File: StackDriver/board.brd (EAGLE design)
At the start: 106.7 x 85.1 mm, 49 parts, among them IC1 LM741P, IC10 LM741P, IC11 LM741P, IC12 LM741P, IC13 LM741P, IC14 LM741P, IC15 LM741P, IC2 LM741P, IC3 LM741P, IC4 LM741P, IC5 LM741P, IC6 LM741P, IC7 LM741P, IC8 LM741P, IC9 LM741P

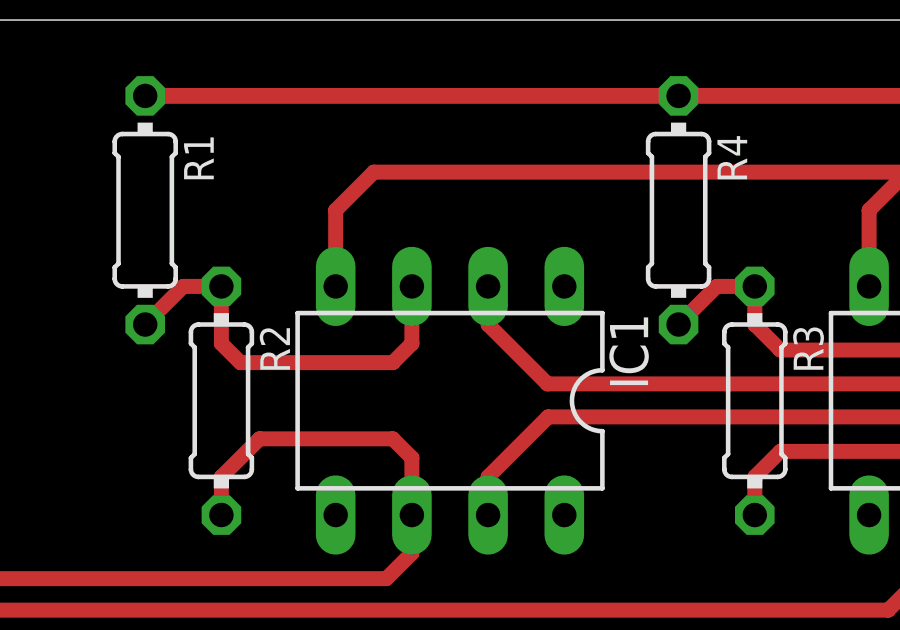
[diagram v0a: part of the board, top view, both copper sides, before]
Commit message: Nie umiem w płytki. Teraz bedzie gut
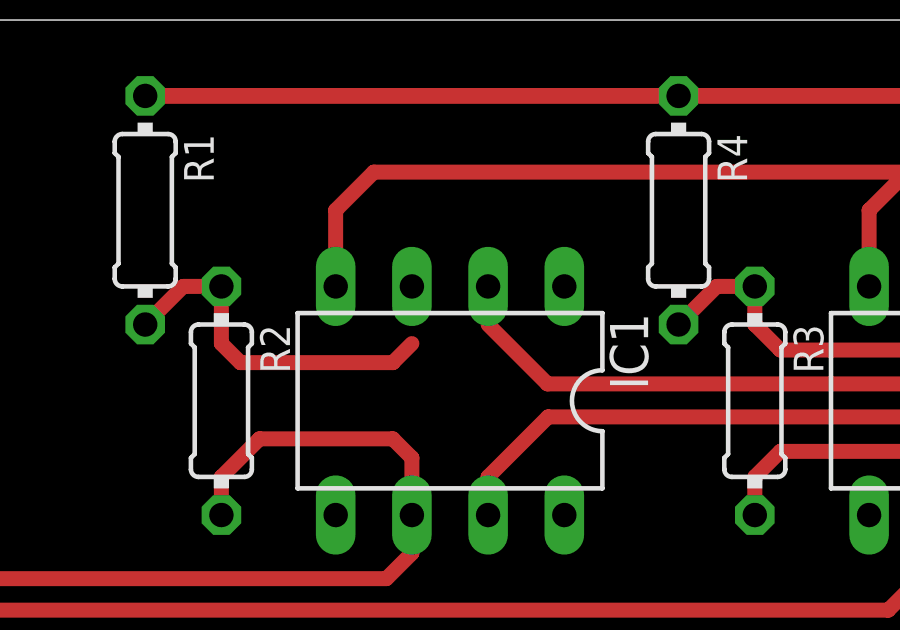
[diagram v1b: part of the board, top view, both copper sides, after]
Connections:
- net N$2: now also IC1.2; no longer IC1.3
- net SYG: now also IC1.3; no longer IC1.2
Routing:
- net N$2: track 13.8 -> 11.8 mm
- net SYG: track 368.1 -> 366.8 mm
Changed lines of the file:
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@@
 <layer number="20" name="Dimension" color="24" fill="1" visible="yes" active="yes"/>
 <layer number="21" name="tPlace" color="7" fill="1" visible="yes" active="yes"/>
-<layer number="22" name="bPlace" color="7" fill="1" visible="no" active="yes"/>
+<layer number="22" name="bPlace" color="7" fill="1" visible="yes" active="yes"/>
 <layer number="23" name="tOrigins" color="15" fill="1" visible="yes" active="yes"/>
-<layer number="24" name="bOrigins" color="15" fill="1" visible="no" active="yes"/>
+<layer number="24" name="bOrigins" color="15" fill="1" visible="yes" active="yes"/>
 <layer number="25" name="tNames" color="7" fill="1" visible="yes" active="yes"/>
-<layer number="26" name="bNames" color="7" fill="1" visible="no" active="yes"/>
-<layer number="27" name="tValues" color="7" fill="1" visible="no" active="yes"/>
-<layer number="28" name="bValues" color="7" fill="1" visible="no" active="yes"/>
+<layer number="26" name="bNames" color="7" fill="1" visible="yes" active="yes"/>
+<layer number="27" name="tValues" color="7" fill="1" visible="yes" active="yes"/>
+<layer number="28" name="bValues" color="7" fill="1" visible="yes" active="yes"/>
 <layer number="29" name="tStop" color="7" fill="3" visible="no" active="yes"/>
 <layer number="30" name="bStop" color="7" fill="6" visible="no" active="yes"/>
@@
 </signal>
 <signal name="N$2">
-<contactref element="IC1" pad="3"/>
 <contactref element="R2" pad="1"/>
 <contactref element="R1" pad="2"/>
 <wire x1="12.7" y1="71.12" x2="13.97" y2="71.12" width="0.5" layer="1"/>
-<wire x1="20.32" y1="71.12" x2="20.32" y2="69.215" width="0.5" layer="1"/>
 <wire x1="20.32" y1="69.215" x2="19.685" y2="68.58" width="0.5" layer="1"/>
 <wire x1="14.605" y1="68.58" x2="13.97" y2="69.215" width="0.5" layer="1"/>
@@
 <wire x1="13.97" y1="69.215" x2="13.97" y2="71.12" width="0.5" layer="1"/>
 <wire x1="11.43" y1="69.85" x2="12.7" y2="71.12" width="0.5" layer="1"/>
+<contactref element="IC1" pad="2"/>
+<wire x1="20.32" y1="69.215" x2="22.86" y2="71.12" width="0" layer="19" extent="1-1"/>
 </signal>
 <signal name="SYG">
-<contactref element="IC1" pad="2"/>
 <contactref element="IC2" pad="2"/>
 <contactref element="IC3" pad="2"/>
@@
 <contactref element="IC15" pad="2"/>
 <contactref element="JP1" pad="3"/>
-<wire x1="22.86" y1="71.12" x2="22.86" y2="69.85" width="0.5" layer="1"/>
 <wire x1="22.86" y1="69.85" x2="24.8392" y2="67.8708" width="0.5" layer="1"/>
 <wire x1="24.8392" y1="67.8708" x2="41.91" y2="67.8708" width="0.5" layer="1"/>
@@
 <wire x1="22.86" y1="24.13" x2="24.7608" y2="22.2292" width="0.5" layer="1"/>
 <wire x1="24.7608" y1="22.2292" x2="41.91" y2="22.2292" width="0.5" layer="1"/>
+<contactref element="IC1" pad="3"/>
+<wire x1="22.86" y1="69.85" x2="20.32" y2="71.12" width="0" layer="19" extent="1-1"/>
 </signal>
 <signal name="GND">
